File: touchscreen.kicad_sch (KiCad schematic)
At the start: 46 parts, among them SW1 0, SW2 SW_SPDT, SW4 0

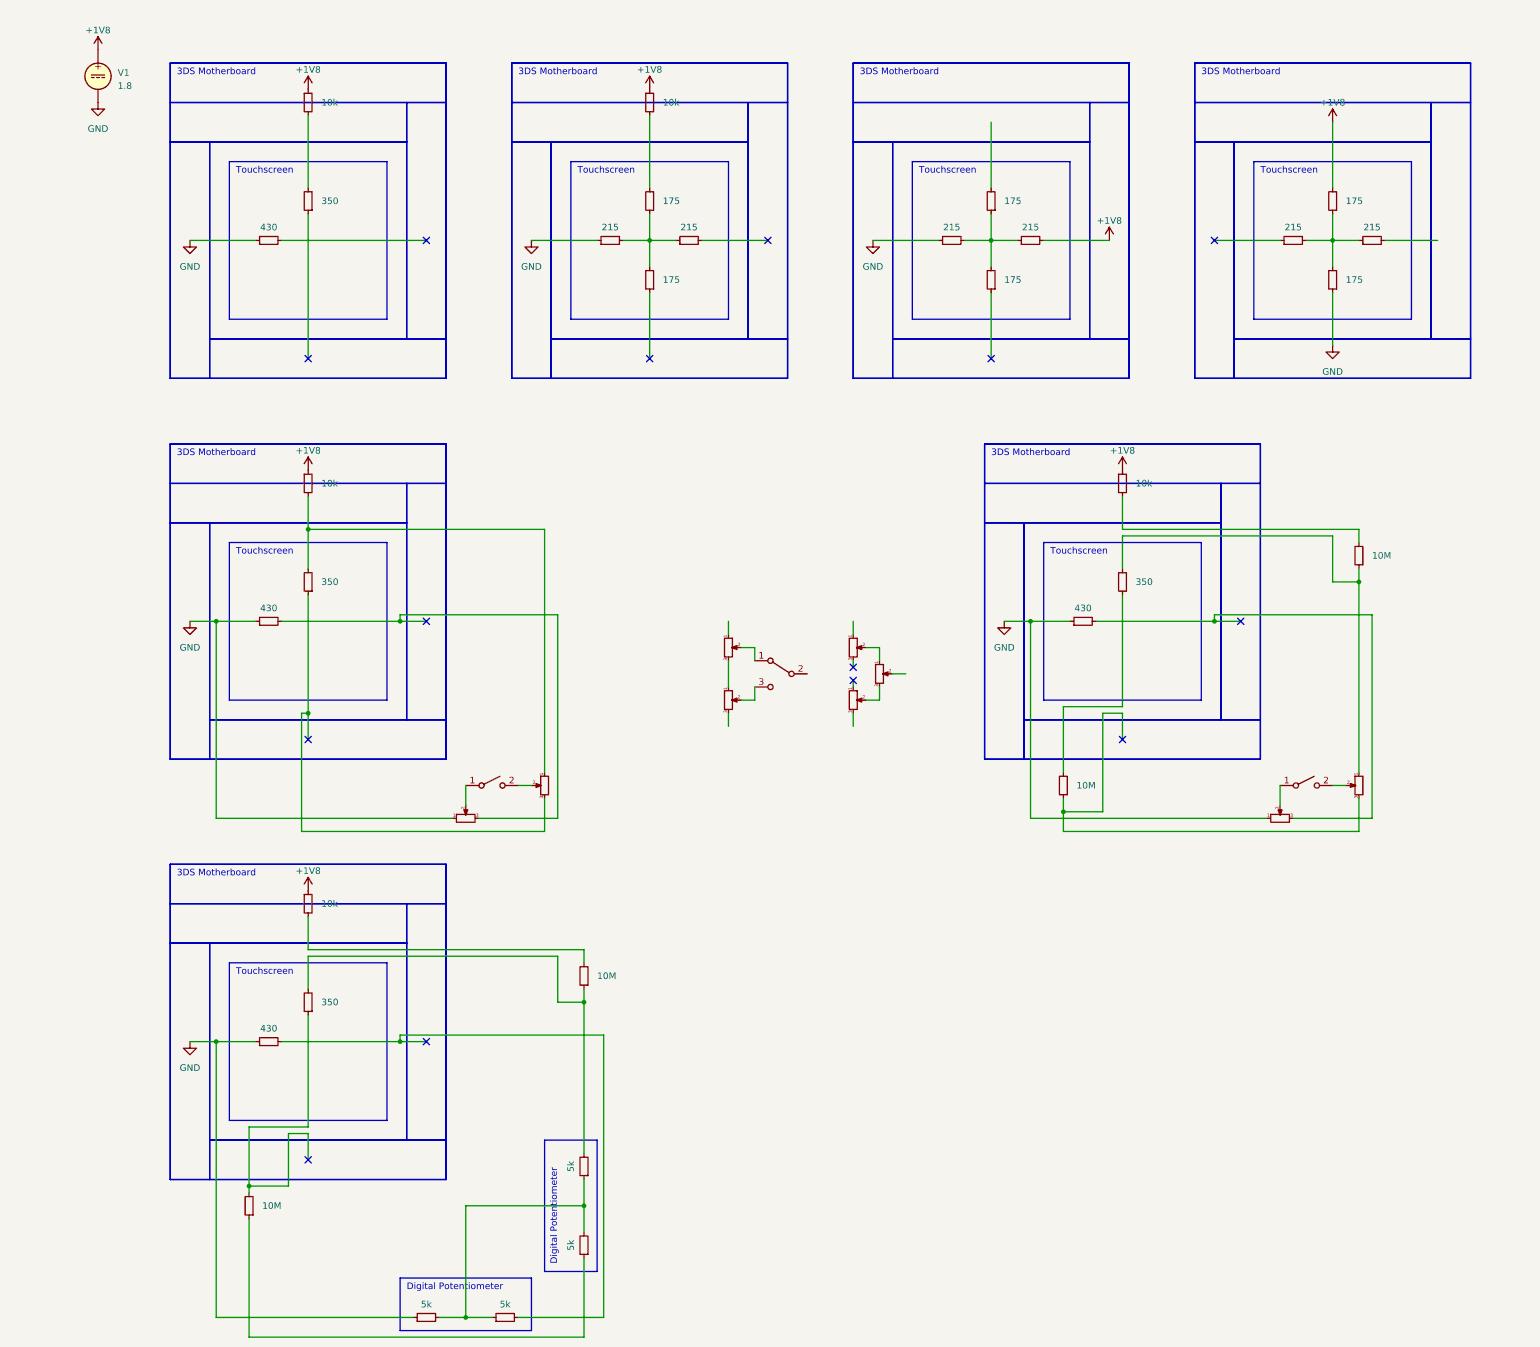
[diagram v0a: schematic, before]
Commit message: Update
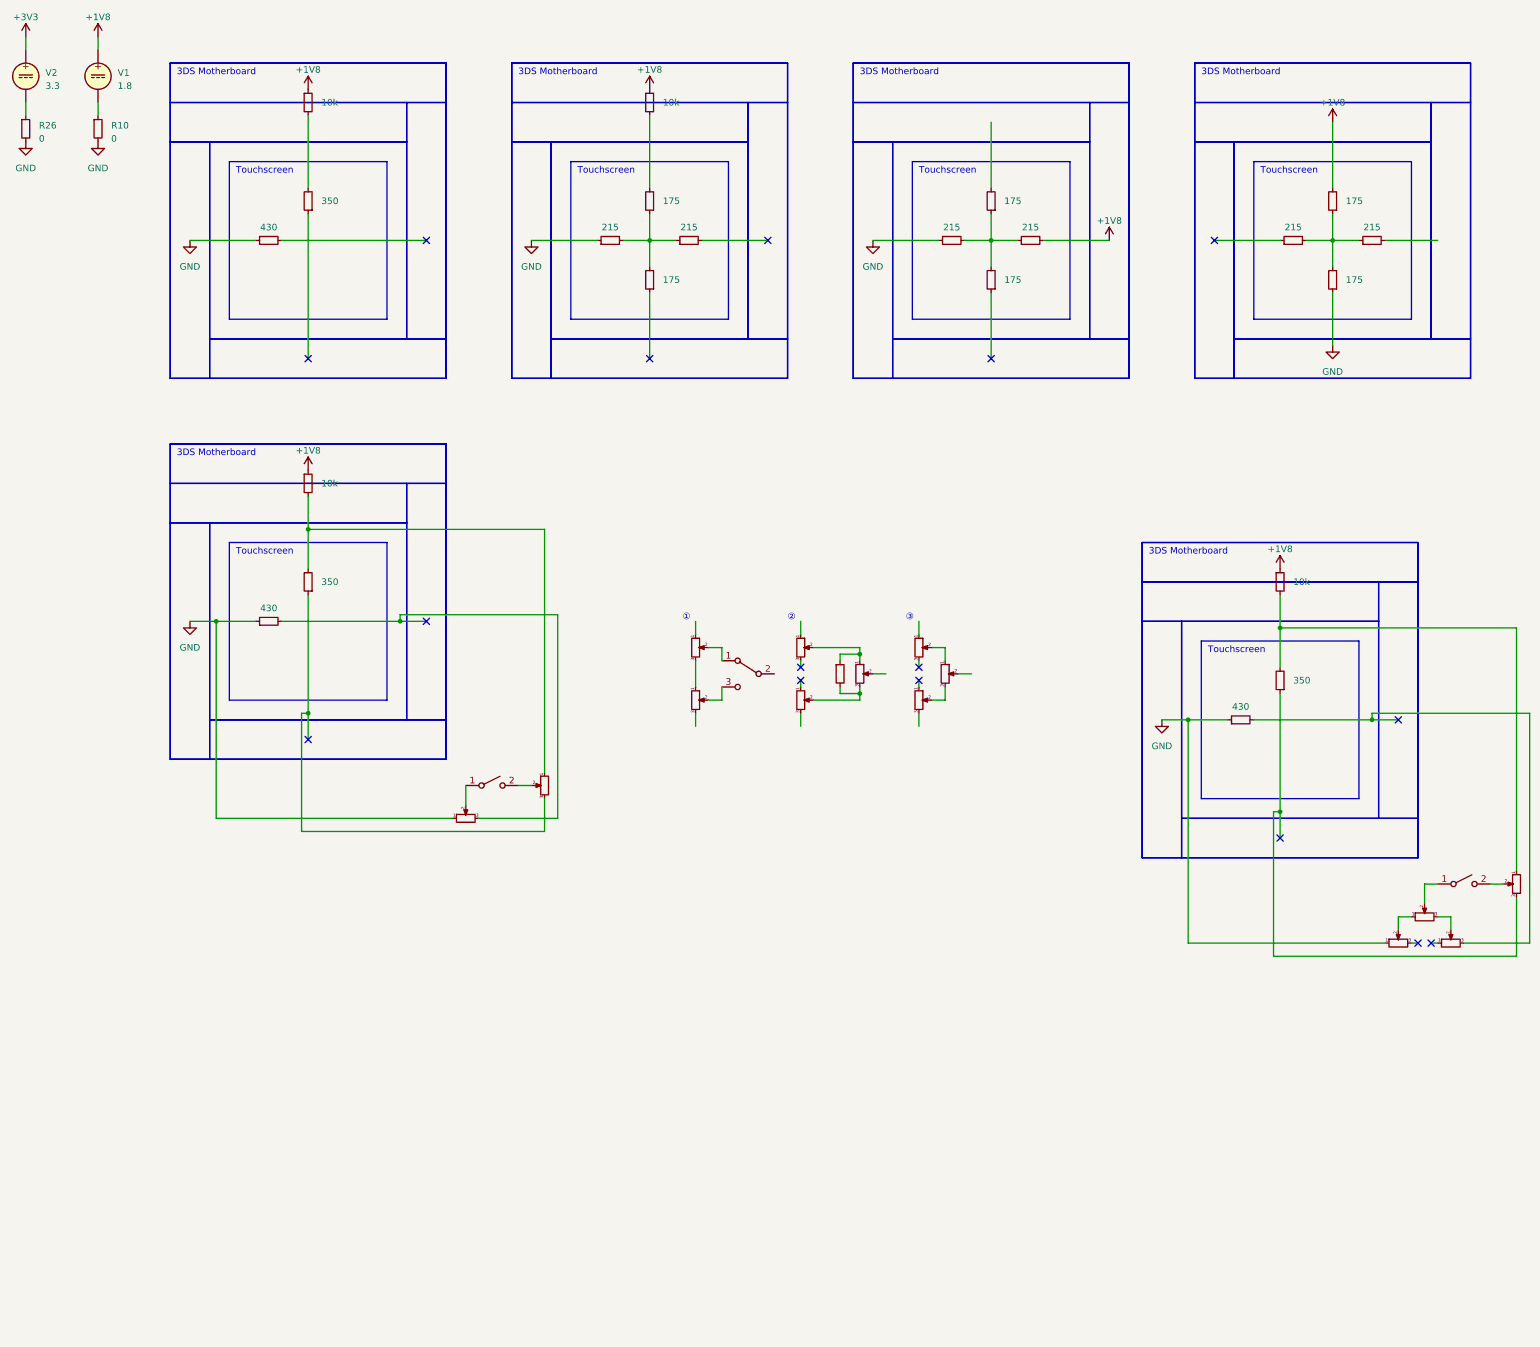
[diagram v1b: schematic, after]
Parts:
- removed R25: 10k, symbol Device:R_Small
- removed R27, R28, R29, R30: 5k, symbol Device:R_Small
- removed R31, R32, R33: 10M, symbol Device:R_Small
- removed RV8: R_Potentiometer_Small, symbol Device:R_Potentiometer_Small
- removed SW4: 0, symbol Switch:SW_SPST
- added RV10, RV11, RV12, RV13, RV14, RV15: R_Potentiometer_Small, symbol Device:R_Potentiometer_Small
- added SW3: 0, symbol Switch:SW_SPST
- added V2: 3.3, symbol Simulation_SPICE:VDC
- R10: value 10M -> 0
- R24: value 430 -> 4.7
- R26: value 350 -> 0
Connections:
- net GND: now also R10.2, R26.2, RV13.1; no longer R24.1, V1.2
- net at R9.1: now also RV9.3
- net at R9.2, RV9.1: now also R8.2; no longer R10.1
- net at R7.2: now also RV14.3
- net at RV9.2: now also SW3.2 (B)
- net at R26.1: now also V2.2
- net at R24.2: now also RV11.2, RV12.3
- new net: RV13.2, RV15.1
- new net: RV15.2, SW3.1 (A)
- new net: RV14.2, RV15.3
- new net: R24.1, RV10.2, RV12.1
- new net: R10.1, V1.2
- new net +3V3: V2.1
- no-connect marks 14 -> 16
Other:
- note added: "①"
- note added: "②"
- note added: "③"
- note removed: "Digital Potentiometer"
